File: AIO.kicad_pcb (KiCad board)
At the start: 2 copper layers, 91 x 78 mm, 359 parts, among them J1 Conn_01x02_MountingPin, J1 JST SH1.0, J1 PH2.0, J1 SH1.0, J1 Sh 1.0, J2 SH1.0, J2 USB_C_Receptacle_PowerOnly_6P, J2 USB_C_Receptacle_USB2.0_16P, J3 JST PH2.0, J3 SH1.0, J3 USB_C_Receptacle_PowerOnly_6P, J3 USB_C_Receptacle_USB2.0_16P, Q1 AO3401A, Q2 AO3400A, Q2 MBT3904DW1, SW1 Boot, SW1 Reset, SW1 SW_Push, SW1 SW_SPDT, SW2 Boot, SW2 Reset, SW2 SW_Push, SW2 SW_SPDT, SW3 Boot, SW3 SW_Push_SPDT, SW3 SW_SPDT, SW3 SW_SPDT_312, U1 AP2112K-3.3, U1 MPU-6050, U1 TP4057, U1 XC6206P182MR, U2 AP2112K-3.3, U2 ESP32-S3-WROOM-1, U2 ESP32-WROOM-32U, U2 IP5306, U2 MPU-6050, U3 ESP32-C3-MINI-1, U3 ESP32C3_SuperMini, U3 MCP73831-2-OT, U3 ME6211C33M5, U3 MPU-9250, U4 AP2112K-3.3, U4 MCP73831-2-OT, U4 MPU-6050, U4 TP4057, U5 ESP32-S2, U5 XC6206P182MR, U6 MPU-9250, Y1 40MHz

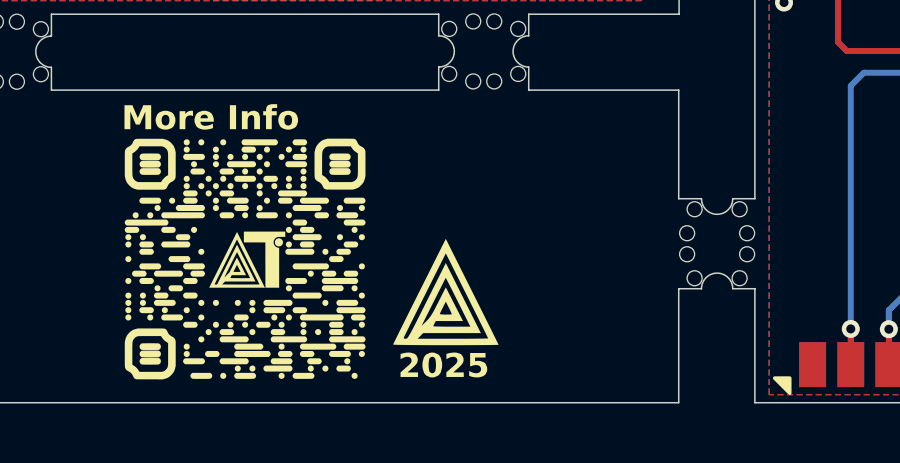
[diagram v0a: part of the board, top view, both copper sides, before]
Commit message: Update AIO.kicad_pcb
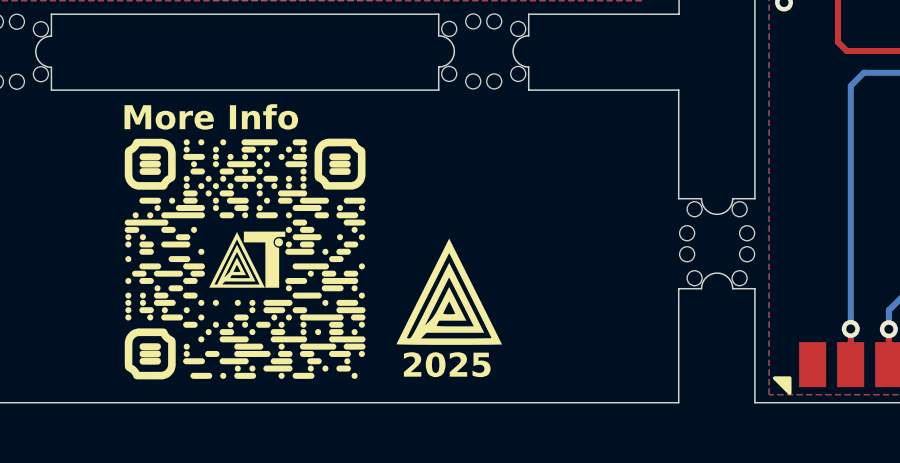
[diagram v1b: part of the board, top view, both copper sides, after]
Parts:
- moved G*** 0.11 mm to (192.2, 126.3) (x2)
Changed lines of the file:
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@@
 	(footprint "LOGO"
 		(layer "F.Cu")
-		(at 192.09 126.36)
+		(at 192.202689 126.349506)
 		(property "Reference" "G***"
 			(at 0 0 0)
@@
 	(footprint "LOGO"
 		(layer "B.Cu")
-		(at 192.06 126.35 180)
+		(at 192.172689 126.339506 180)
 		(property "Reference" "G***"
 			(at 0 0 0)
@@
 	)
 	(gr_text "2025"
-		(at 193.67 129.36 -0)
+		(at 193.782689 129.349506 -0)
 		(layer "B.SilkS")
 		(effects
@@
 	)
 	(gr_text "2025"
-		(at 190.48 129.37 0)
+		(at 190.592689 129.359506 0)
 		(layer "F.SilkS")
 		(effects
